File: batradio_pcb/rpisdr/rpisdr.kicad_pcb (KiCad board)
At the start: 2 copper layers, 65 x 56 mm, 71 parts, among them J1 RPI_header, J2 Conn_01x03, J3 Conn_01x03, U1 ldln025, U2 mcp33131, U3 ldln025, U4 ths4521, U5 lmh6629, U6 lmh6629, U7 ldln025, U8 MCP4821

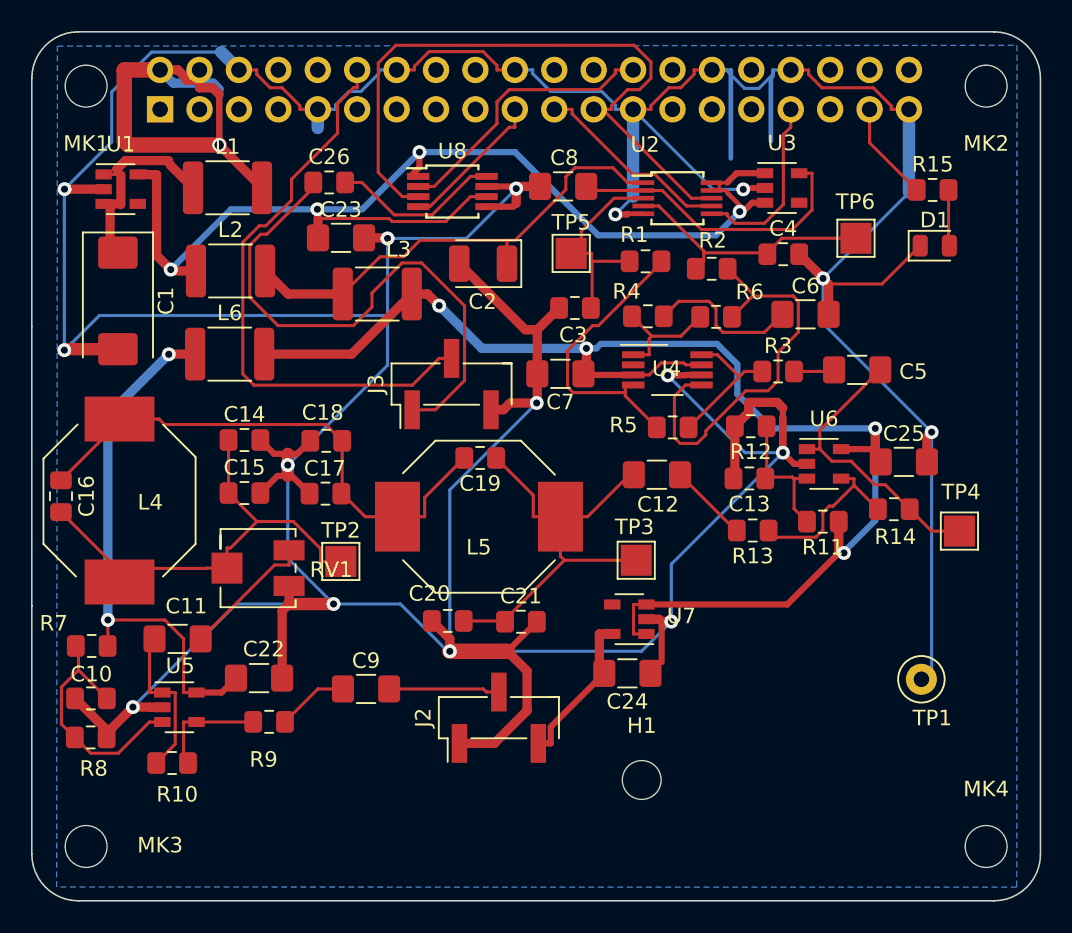
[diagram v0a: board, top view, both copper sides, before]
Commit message: Updated README
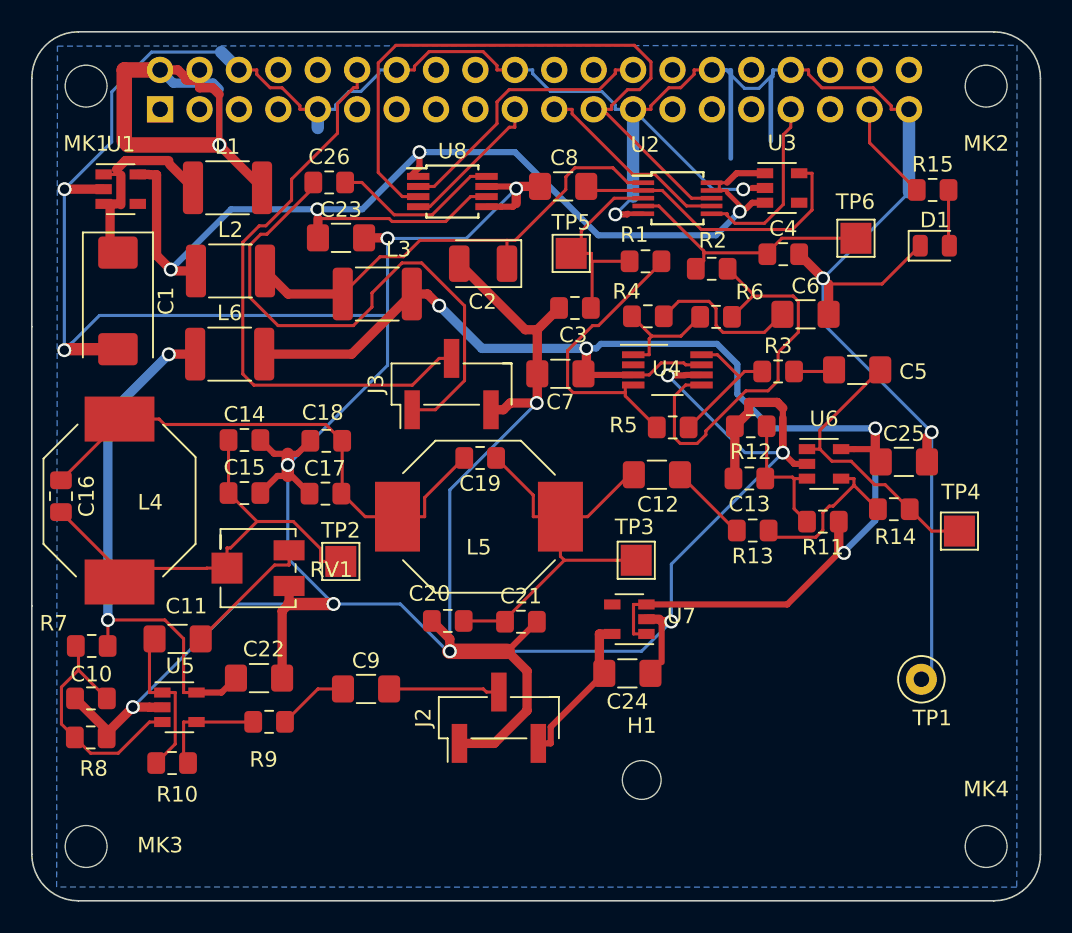
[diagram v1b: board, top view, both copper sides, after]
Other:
- net class Default removed
- net class Power removed
